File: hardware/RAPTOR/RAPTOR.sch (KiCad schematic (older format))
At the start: 48 parts, among them J1 SOLC_CONN, J2 SOLP_CONN, J3 JST_2MM_MALE, J4 CONN_LED_FIX, J5 CONN_SOLP_LED, J6 CONN_SOLC_LED, P1 Power, P2 Analog, P3 Digital, P4 Digital, P5 CONN_01X01, P6 CONN_01X01, P7 CONN_01X01, P8 CONN_01X01, Q1 MOSFET-NCH-2N7002PW, Q2 MOSFET-NCH-2N7002PW, Q3 MOSFET-NCH-2N7002PW, Q4 MOSFET-NCH-2N7002PW, SW1 EEPROM_BTN, SW2 SOLC_SW, SW3 SOLP_SW, U1 BMP280 Breakout, U2 BNO055 Breakout, U3 OpenLog, U4 AdafruitGPS, U5 U3V12F12, U6 L4940V5

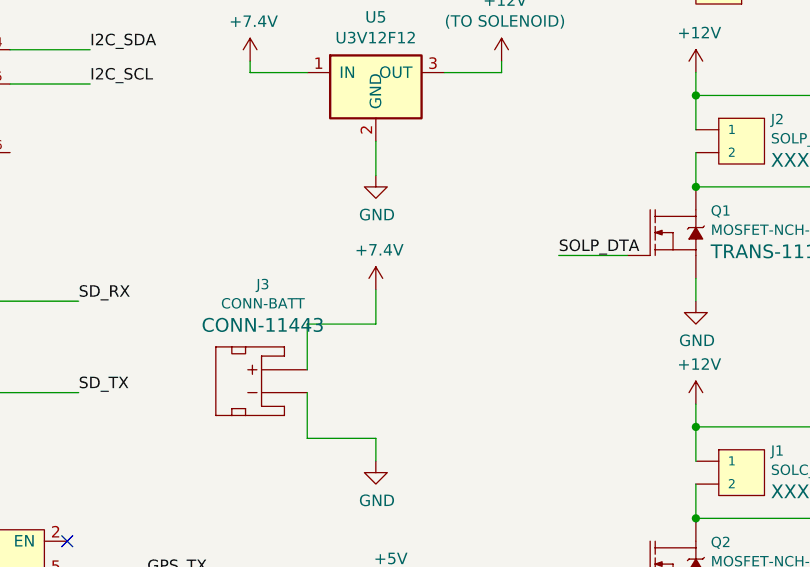
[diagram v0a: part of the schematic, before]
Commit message: add RBF
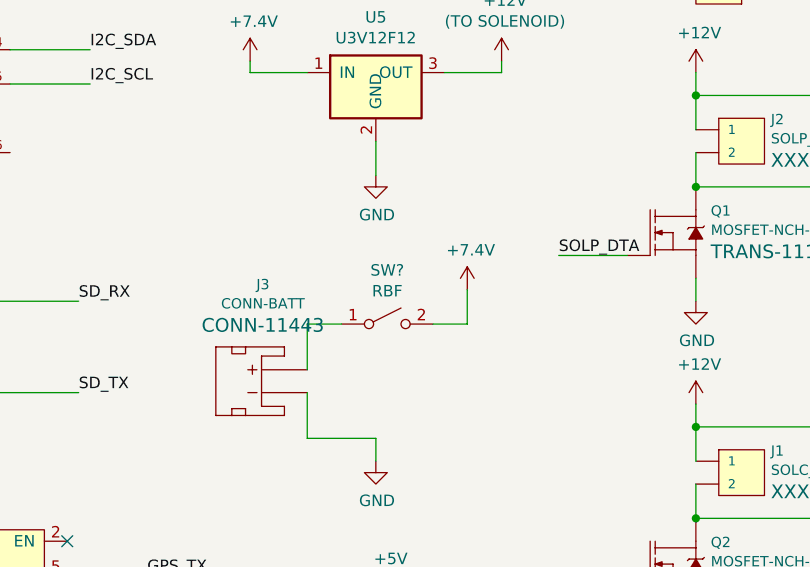
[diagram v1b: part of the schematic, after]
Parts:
- added SW?: RBF, symbol Switch:SW_SPST
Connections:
- net +7.5V: now also SW?.2 (B); no longer J3.2 (+)
- new net: J3.2 (+), SW?.1 (A)
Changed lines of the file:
@@
 L power:+7.5V #PWR015
 U 1 1 5C4F2CBE
-P 3550 3050
-F 0 "#PWR015" H 3550 2900 50  0001 C CNN
-F 1 "+7.5V" H 3565 3223 50  0001 C CNN
-F 2 "" H 3550 3050 50  0001 C CNN
-F 3 "" H 3550 3050 50  0001 C CNN
-F 4 "+7.4V" H 3565 3223 50  0000 C CNN "Real Value"
-	1    3550 3050
-	1    0    0    -1
-$EndComp
-Wire Wire Line
-	3550 3050 3550 3200
+P 3950 3050
+F 0 "#PWR015" H 3950 2900 50  0001 C CNN
+F 1 "+7.5V" H 3965 3223 50  0001 C CNN
+F 2 "" H 3950 3050 50  0001 C CNN
+F 3 "" H 3950 3050 50  0001 C CNN
+F 4 "+7.4V" H 3965 3223 50  0000 C CNN "Real Value"
+	1    3950 3050
+	1    0    0    -1
+$EndComp
+Wire Wire Line
+	3950 3050 3950 3200
 $Comp
 L power:GND #PWR09
@@
 	3550 3700 3550 3800
 Wire Wire Line
-	3550 3200 3250 3200
-Wire Wire Line
 	3250 3200 3250 3400
 Wire Wire Line
@@
 	1    0    0    -1
 $EndComp
+$Comp
+L Switch:SW_SPST SW?
+U 1 1 5C4BDD6E
+P 3600 3200
+F 0 "SW?" H 3600 3435 50  0000 C CNN
+F 1 "RBF" H 3600 3344 50  0000 C CNN
+F 2 "" H 3600 3200 50  0001 C CNN
+F 3 "" H 3600 3200 50  0001 C CNN
+	1    3600 3200
+	1    0    0    -1
+$EndComp
+Wire Wire Line
+	3250 3200 3400 3200
+Wire Wire Line
+	3800 3200 3950 3200
 $EndSCHEMATC
